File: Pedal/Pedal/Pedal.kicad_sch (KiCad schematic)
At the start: 22 parts, among them J1 Conn_01x02, J2 Conn_01x02, U1 YAAJ_BluePill_Part_Like, U2 MCP2561-E-SN, U3 AP63200WU

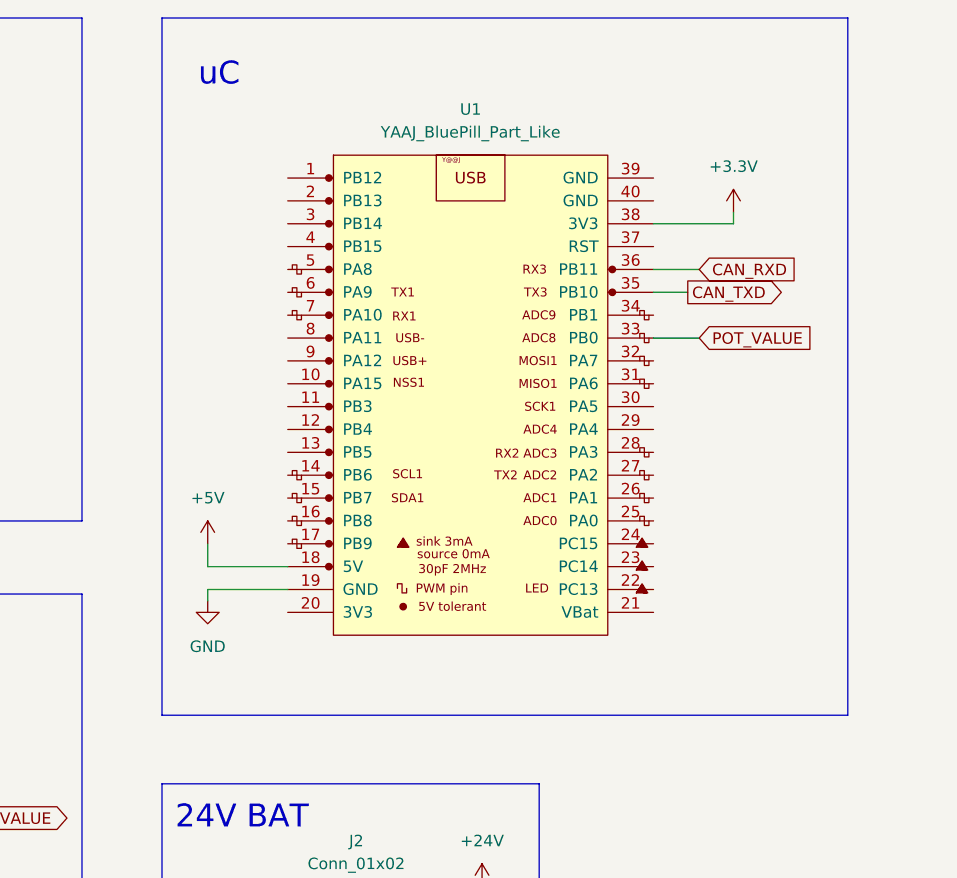
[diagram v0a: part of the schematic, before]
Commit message: lista la placa para imprimir
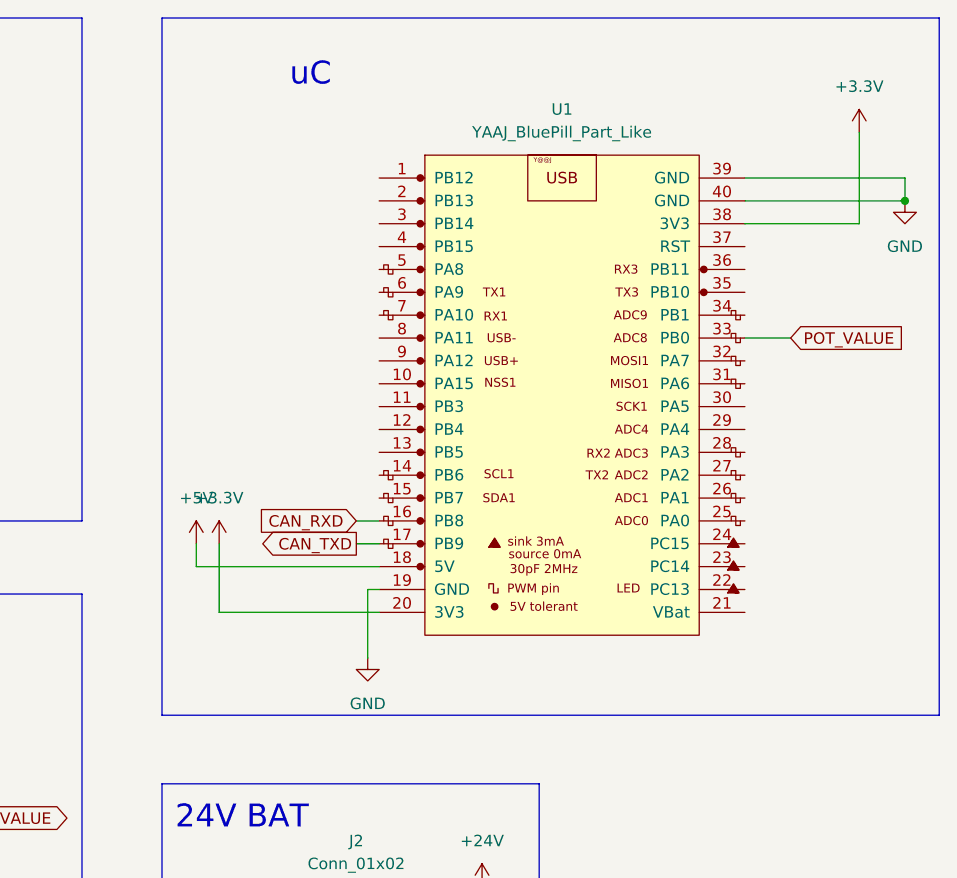
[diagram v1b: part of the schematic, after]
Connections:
- net +3.3V: now also U1.20 (3V3)
- net CAN_RXD: now also U1.16 (PB8); no longer U1.36 (PB11)
- net CAN_TXD: now also U1.17 (PB9); no longer U1.35 (PB10)
- net GND: now also U1.39 (GND), U1.40 (GND)
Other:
- moved on the sheet: U1
